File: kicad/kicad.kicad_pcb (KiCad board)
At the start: 2 copper layers, 47.5 x 52 mm, 18 parts, among them J1 switch, SW2 button, SW3 button, SW4 button, U1 ESP-12F, U2 AMS1117-3.3

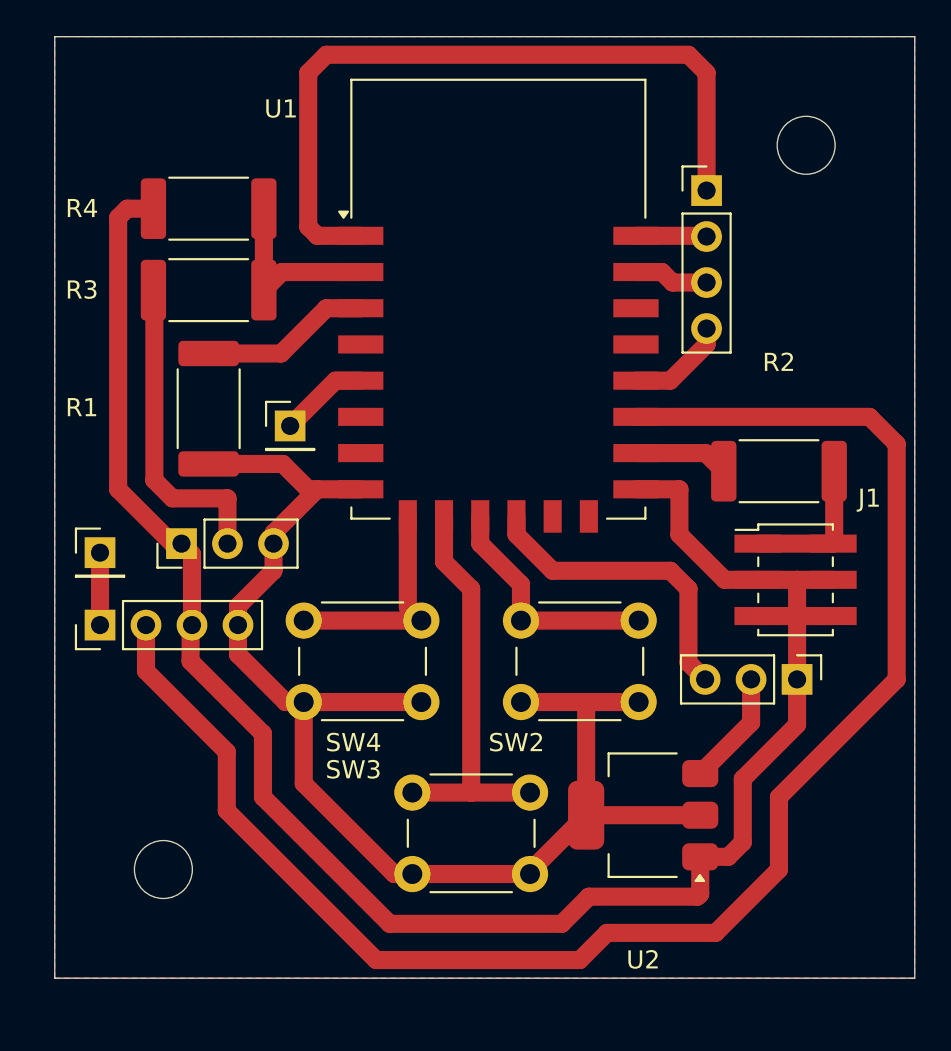
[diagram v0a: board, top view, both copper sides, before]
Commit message: updated frontend backend, improved cpp, added admin panel
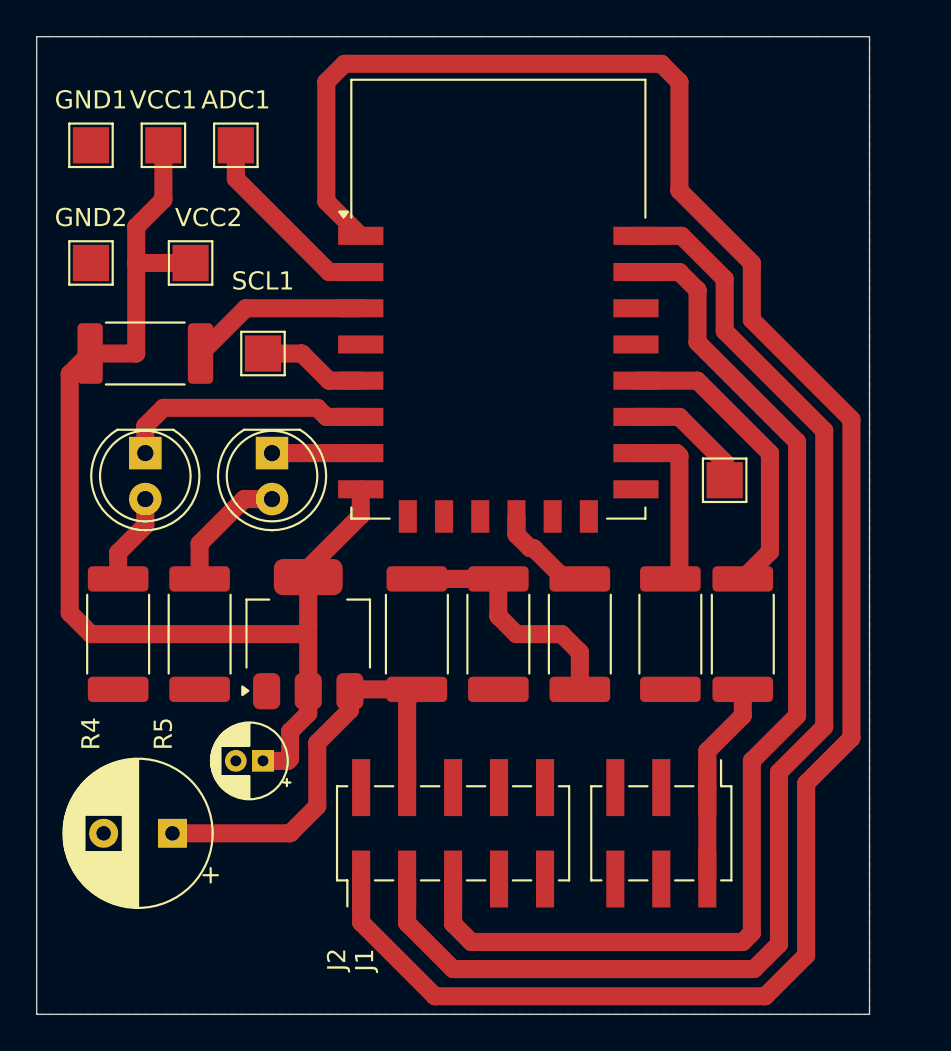
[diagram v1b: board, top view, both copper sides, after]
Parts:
- removed REF** (x2): PinHeader_1x04_P2.54mm_Vertical, Connector_PinHeader_2.54mm:PinHeader_1x04_P2.54mm_Vertical
- removed REF** (x2): PinHeader_1x03_P2.54mm_Vertical, Connector_PinHeader_2.54mm:PinHeader_1x03_P2.54mm_Vertical
- removed REF** (x2): MountingHole_3.2mm, MountingHole:MountingHole_3.2mm_M3_ISO7380
- removed REF** (x2): PinHeader_1x01_P2.54mm_Vertical, Connector_PinHeader_2.54mm:PinHeader_1x01_P2.54mm_Vertical
- removed SW2, SW3, SW4: button, Button_Switch_THT:SW_PUSH_6mm_H4.3mm
- added ADC1: OUT, TestPoint:TestPoint_Pad_2.0x2.0mm, F.Cu at (117.5, 80.5)
- added C1: 10V 1000UF, Capacitor_THT:CP_Radial_D8.0mm_P3.80mm, F.Cu at (114.0, 118.5)
- added C2: 10v 47UF, Capacitor_THT:CP_Radial_D4.0mm_P1.50mm, F.Cu at (119.0, 114.5)
- added D1: LED, LED_THT:LED_D5.0mm, F.Cu at (112.5, 97.5)
- added D2: LED, LED_THT:LED_D5.0mm, F.Cu at (119.5, 97.5)
- added GND1: OUT, TestPoint:TestPoint_Pad_2.0x2.0mm, F.Cu at (109.5, 80.5)
- added GND2: OUT, TestPoint:TestPoint_Pad_2.0x2.0mm, F.Cu at (109.5, 87.0)
- added J2: input, Connector_PinHeader_2.54mm:PinHeader_2x05_P2.54mm_Vertical_SMD, F.Cu at (129.5, 118.5)
- added R5: 200, Resistor_SMD:R_2512_6332Metric_Pad1.40x3.35mm_HandSolder, F.Cu at (115.5, 107.5)
- added R6: idk, Resistor_SMD:R_2512_6332Metric_Pad1.40x3.35mm_HandSolder, F.Cu at (127.5, 107.5)
- added R7: idk, Resistor_SMD:R_2512_6332Metric_Pad1.40x3.35mm_HandSolder, F.Cu at (132.0, 107.5)
- added R8: 10k, Resistor_SMD:R_2512_6332Metric_Pad1.40x3.35mm_HandSolder, F.Cu at (136.5, 107.5)
- added SCL1: OUT, TestPoint:TestPoint_Pad_2.0x2.0mm, F.Cu at (119.0, 92.0)
- added SDA1: OUT, TestPoint:TestPoint_Pad_2.0x2.0mm, F.Cu at (144.5, 99.0)
- added VCC1: OUT, TestPoint:TestPoint_Pad_2.0x2.0mm, F.Cu at (113.5, 80.5)
- added VCC2: OUT, TestPoint:TestPoint_Pad_2.0x2.0mm, F.Cu at (115.0, 87.0)
- J1: value switch -> Boot Switch; footprint Connector_PinHeader_2.00mm:PinHeader_2x03_P2.00mm_Vertical_SMD -> Connector_PinHeader_2.54mm:PinHeader_2x03_P2.54mm_Vertical_SMD
- R3: value 220 -> 10k
- R4: value 100 -> 200
- moved R3 35.1 mm to (145.5, 107.5), turned to 90 degrees
- moved R4 24.0 mm to (111.0, 107.5), turned to 90 degrees
- moved U2 21.0 mm to (121.5, 107.5), turned to 90 degrees
- moved J1 15.8 mm to (141.0, 118.5), turned to -90 degrees
- moved R2 10.8 mm to (141.5, 107.5), turned to -90 degrees
- moved R1 4.64 mm to (112.5, 92.0), turned to 0 degrees
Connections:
- J1 pad 1: Net-(J1-Pin_a1) -> Net-(J1-Pin_1)
- J1 pad 2: Net-(J1-Pin_a1) -> -BATT
- J1 pad 3: GND -> -BATT
- J1 pad 4: GND -> Net-(J1-Pin_1)
- J1 pad 5: GND -> -BATT
- J1 pad 6: GND -> -BATT
- R1 pad 1: Net-(U1-EN) -> Net-(U1-VCC)
- R1 pad 2: VCC -> Net-(U1-EN)
- R2 pad 2: Net-(J1-Pin_a1) -> -BATT
- R3 pad 1: ADC -> Net-(J1-Pin_1)
- R3 pad 2: Net-(U1-ADC) -> Net-(U1-GPIO0)
- R4 pad 1: GND -> -BATT
- R4 pad 2: Net-(U1-ADC) -> Net-(D1-A)
- U1 pad 10: Net-(U1-MISO) -> unconnected-(U1-MISO-Pad10)
- U1 pad 11: Net-(U1-GPIO9) -> unconnected-(U1-GPIO9-Pad11)
- U1 pad 12: SIG -> Net-(U1-GPIO10)
- U1 pad 15: GND -> -BATT
- U1 pad 17: SDA -> Net-(U1-GPIO2)
- U1 pad 18: IO 0 -> Net-(U1-GPIO0)
- U1 pad 5: SCL -> Net-(U1-GPIO14)
- U1 pad 6: unconnected-(U1-GPIO12-Pad6) -> Net-(D1-K)
- U1 pad 7: unconnected-(U1-GPIO13-Pad7) -> Net-(D2-K)
- U1 pad 8: VCC -> Net-(U1-VCC)
- U1 pad 9: Net-(U1-CS0) -> unconnected-(U1-CS0-Pad9)
- U2 pad 1: GND -> -BATT
- U2 pad 2: VCC -> Net-(U1-VCC)
- U2 pad 3: VIN -> +BATT
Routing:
- net GND: track 104.6 -> 0.00 mm
- net SDA: track 89.3 -> 0.00 mm
- net VCC: track 73.9 -> 0.00 mm
- net RESET: track 40.9 -> 112.4 mm
- net TX: track 3.92 -> 70.5 mm
- net Net-(U1-VCC): track 0.00 -> 64.5 mm
- net RX: track 4.14 -> 62.2 mm
- net +BATT: track 0.00 -> 25.1 mm
- net Net-(U1-MISO): track 22.4 -> 0.00 mm
- net ADC: track 17.5 -> 0.00 mm
- net SIG: track 17.1 -> 0.00 mm
- net Net-(U1-GPIO0): track 0.00 -> 16.6 mm
- net Net-(D1-K): track 0.00 -> 14.0 mm
- net Net-(R6-Pad2): track 0.00 -> 13.9 mm
- net Net-(U1-GPIO9): track 13.2 -> 0.00 mm
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- added copper zone on F.Cu, net -BATT
- removed copper zone on F.Cu, net GND
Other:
- board size 47.5 x 52 mm -> 46 x 54 mm
